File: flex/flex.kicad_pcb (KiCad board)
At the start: 2 copper layers, 47.2 x 41.5 mm, 18 parts, among them J1 Conn_01x06_Female, J2 Conn_01x03_Female, SW19 SW_Push, SW5 SW_Push, SW9 SW_Push

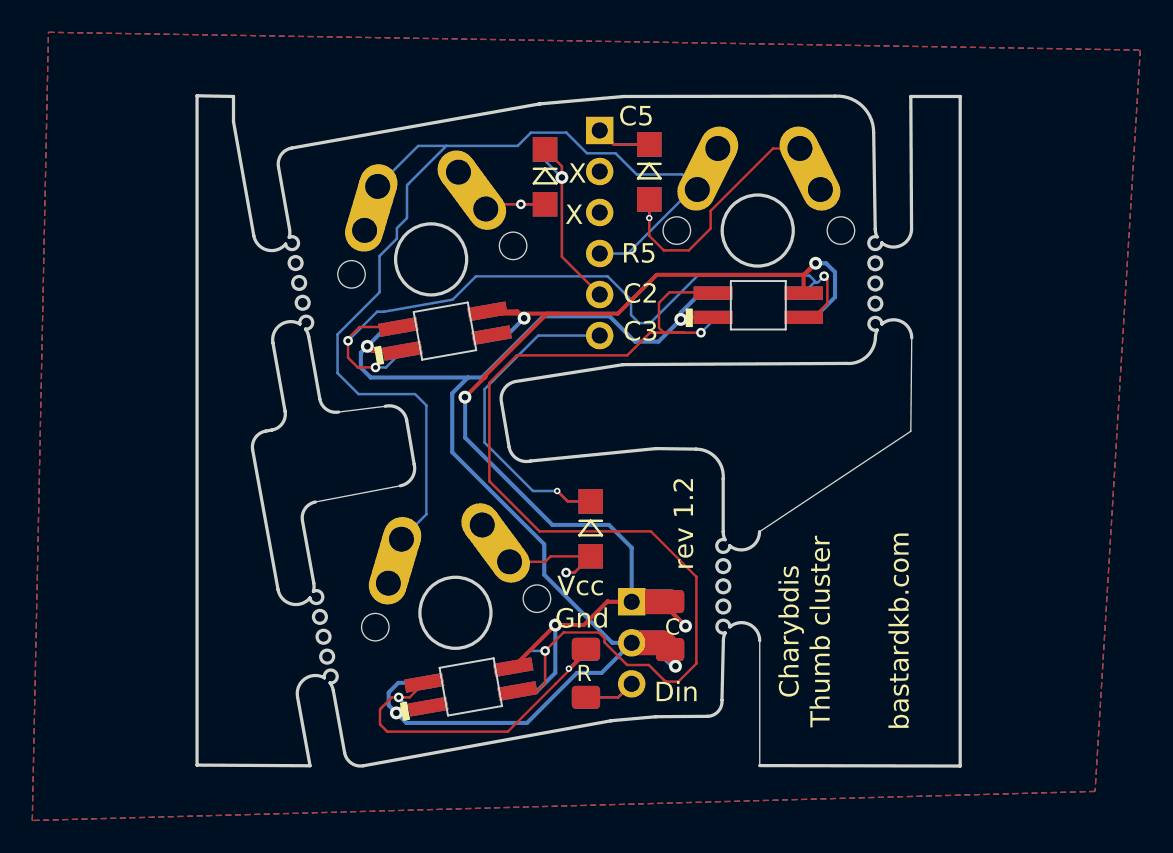
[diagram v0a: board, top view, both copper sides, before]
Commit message: make universal
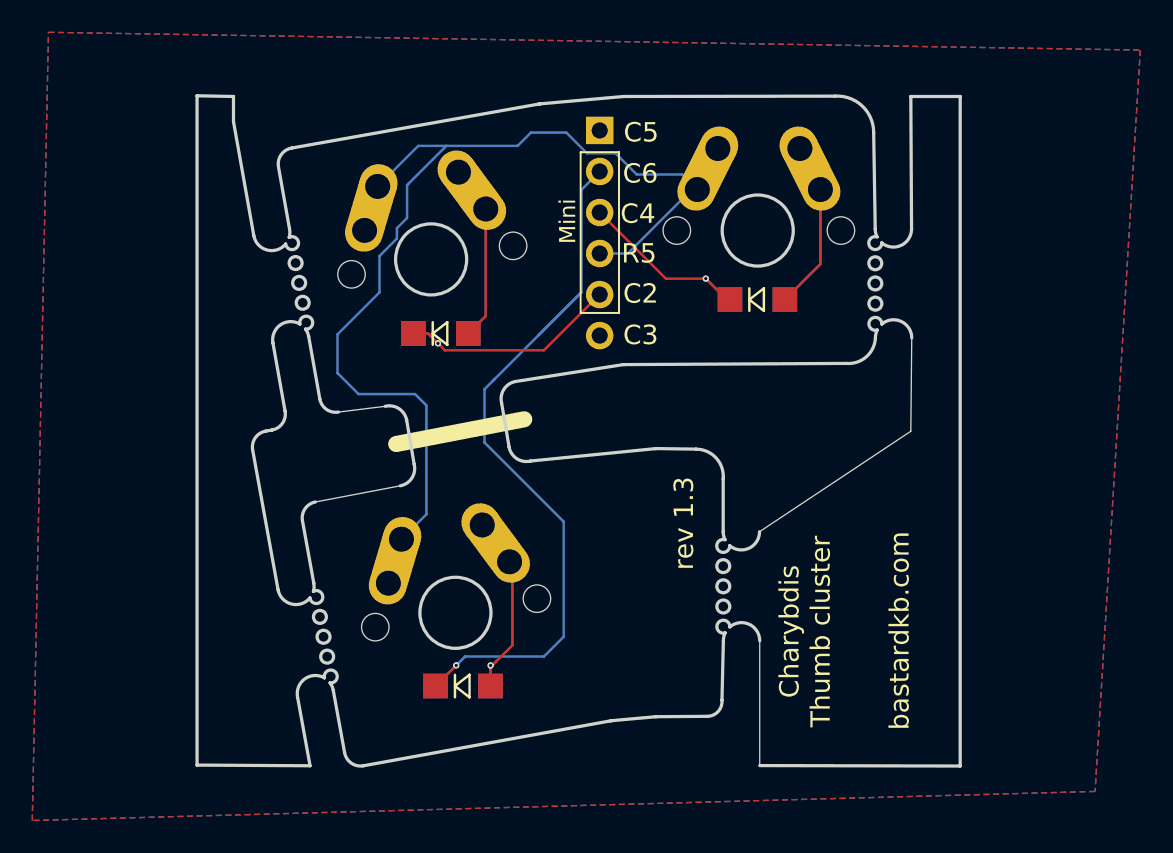
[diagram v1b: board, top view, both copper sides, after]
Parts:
- removed C1, C2: C, LED_SMD:LED_1206_3216Metric_Pad1.42x1.75mm_HandSolder
- removed D10, D12, D2: SK6812MINI, libs2:YS-SK6812MINI-E_REVERSE
- removed D11, D13, D3: SK6812MINI, libs2:YS-SK6812MINI-E_REVERSE_NO_EDGECUT
- removed J2: Conn_01x03_Female, Connector_PinHeader_2.54mm:PinHeader_1x03_P2.54mm_Vertical
- removed R1, R2: R, Resistor_SMD:R_1206_3216Metric_Pad1.42x1.75mm_HandSolder
- moved D9 19.6 mm to (71.0, 102.8), turned to 0 degrees
- moved D5 18.6 mm to (69.6, 81.0), turned to 0 degrees
- moved D19 13.0 mm to (89.2, 78.8), turned to 0 degrees
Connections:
- D19 pad 1: col5 -> col4
- D9 pad 1: col3 -> col6
- J1 pad 1: col5 -> unconnected-(J1-Pad1)
- J1 pad 6: col3 -> unconnected-(J1-Pad6)
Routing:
- net Gnd: track 87.6 -> 0.00 mm, vias 4 -> 0
- net Vcc: track 85.4 -> 0.00 mm, vias 5 -> 0
- net Net-(D2-Pad1): track 67.4 -> 0.00 mm, vias 2 -> 0
- net col6: track 0.00 -> 48.7 mm, vias 0 -> 1
- net Net-(D10-Pad1): track 47.5 -> 0.00 mm, vias 3 -> 0
- net Net-(D2-Pad3): track 24.9 -> 0.00 mm, vias 2 -> 0
- net col3: track 22.5 -> 0.00 mm, vias 1 -> 0
- net col4: track 0.00 -> 12.3 mm, vias 0 -> 1
- net Net-(D5-Pad2): track 5.29 -> 16.3 mm, vias 1 -> 0
- net col5: track 6.86 -> 0.00 mm
- net Din: track 6.35 -> 0.00 mm
- net col2: track 12.6 -> 15.2 mm
- net Net-(D9-Pad2): track 9.04 -> 10.1 mm
- net Net-(D19-Pad2): track 16.4 -> 15.5 mm, vias 1 -> 0
- added copper zone on B.Cu, net (none)
- added copper zone on F.Cu, net (none)
- removed copper zone on B.Cu, net Gnd
- removed copper zone on F.Cu, net Gnd
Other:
- board text added: "C4"
- board text added: "C6"
- board text added: "Mini"
- board text added: "rev 1.3"
- board text removed: "C"
- board text removed: "Din"
- board text removed: "Gnd"
- board text removed: "R"
- board text removed: "Vcc"
- board text removed: "X"
- board text removed: "rev 1.2"
